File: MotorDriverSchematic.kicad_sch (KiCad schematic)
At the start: 5 parts, among them J1 Conn_01x02, J2 Conn_02x20_Odd_Even, J3 Conn_01x02, J4 Conn_01x02, U1 ULN2803A

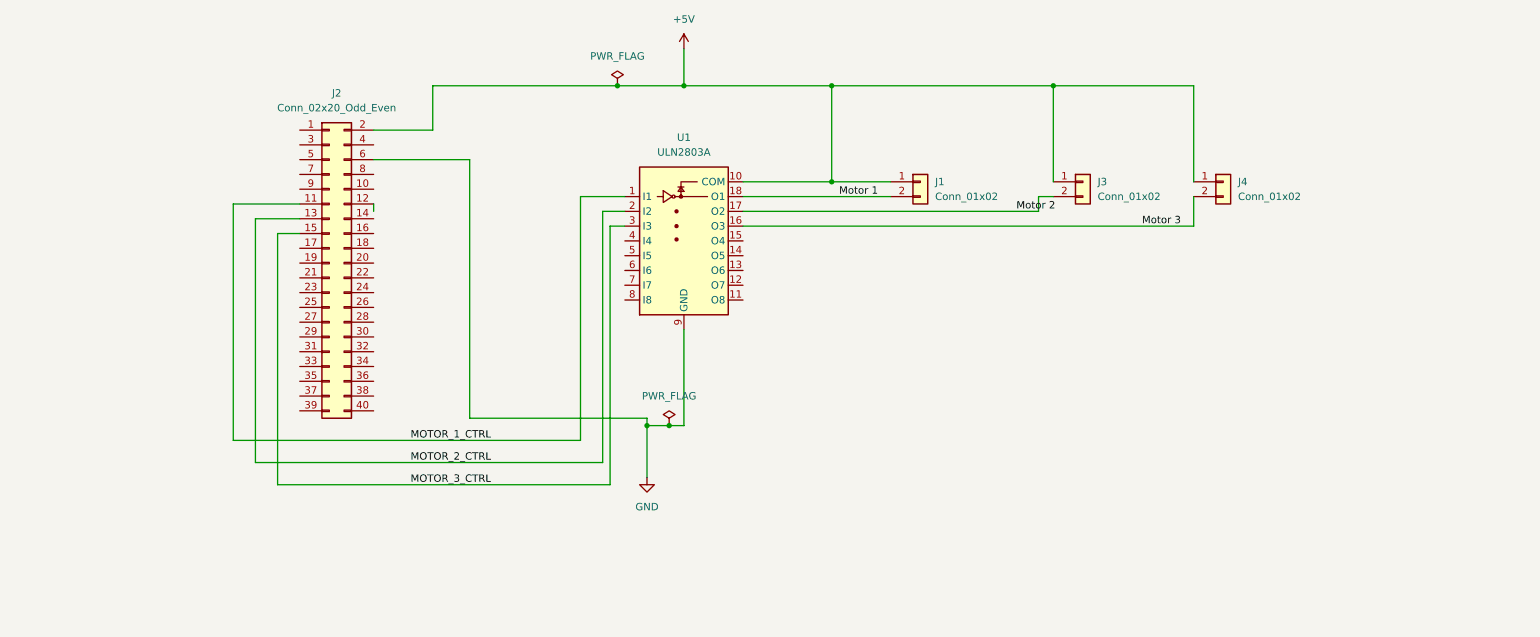
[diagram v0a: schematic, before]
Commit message: Add files via upload
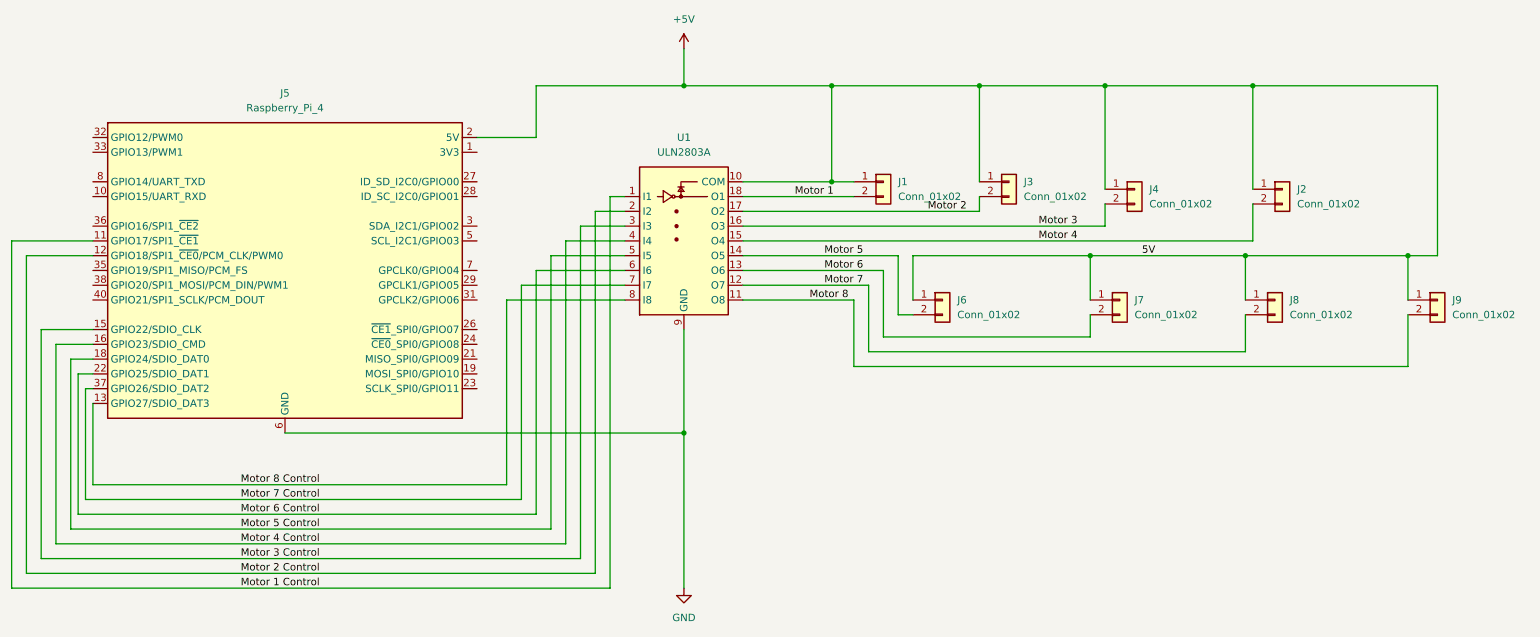
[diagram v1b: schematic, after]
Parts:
- removed J2: Conn_02x20_Odd_Even, symbol Connector_Generic:Conn_02x20_Odd_Even
- added J2, J6, J7, J8, J9: Conn_01x02, symbol Connector_Generic:Conn_01x02
- added J5: Raspberry_Pi_4, symbol Connector:Raspberry_Pi_4
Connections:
- net +5V: now also J2.1 (Pin_1), J5.2 (5V), J5.4 (5V), J6.1 (Pin_1), J7.1 (Pin_1), J8.1 (Pin_1), J9.1 (Pin_1)
- net GND: now also J5.14 (GND), J5.20 (GND), J5.25 (GND), J5.30 (GND), J5.34 (GND), J5.39 (GND), J5.6 (GND), J5.9 (GND)
- net Motor 8: now reaches U1.11 (O8)
- net Motor 8: now also J9.2 (Pin_2)
- net Motor 7: now reaches U1.12 (O7)
- net Motor 7: now also J8.2 (Pin_2)
- net Motor 6: now reaches U1.13 (O6)
- net Motor 6: now also J7.2 (Pin_2)
- net Motor 5: now reaches U1.14 (O5)
- net Motor 5: now also J6.2 (Pin_2)
- net Motor 4: now reaches U1.15 (O4)
- net Motor 4: now also J2.2 (Pin_2)
- net Motor 4 Control: now reaches U1.4 (I4)
- net Motor 4 Control: now also J5.16 (GPIO23/SDIO_CMD)
- net Motor 5 Control: now reaches U1.5 (I5)
- net Motor 5 Control: now also J5.18 (GPIO24/SDIO_DAT0)
- net Motor 6 Control: now reaches U1.6 (I6)
- net Motor 6 Control: now also J5.22 (GPIO25/SDIO_DAT1)
- net Motor 7 Control: now reaches U1.7 (I7)
- net Motor 7 Control: now also J5.37 (GPIO26/SDIO_DAT2)
- net Motor 8 Control: now reaches U1.8 (I8)
- net Motor 8 Control: now also J5.13 (GPIO27/SDIO_DAT3)
- net MOTOR_1_CTRL renamed Motor 1 Control
- net Motor 1 Control: now also J5.11 (GPIO17/SPI1_~{CE1})
- net MOTOR_2_CTRL renamed Motor 2 Control
- net Motor 2 Control: now also J5.12 (GPIO18/SPI1_~{CE0}/PCM_CLK/PWM0)
- net MOTOR_3_CTRL renamed Motor 3 Control
- net Motor 3 Control: now also J5.15 (GPIO22/SDIO_CLK)
- new net: J5.1 (3V3), J5.17 (3V3)
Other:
- moved on the sheet: J1, J3, J4
